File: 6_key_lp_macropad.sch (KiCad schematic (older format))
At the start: 9 parts, among them SW1 Rotary_Encoder_Switch, SW2 SW_Push, U1 ProMicro

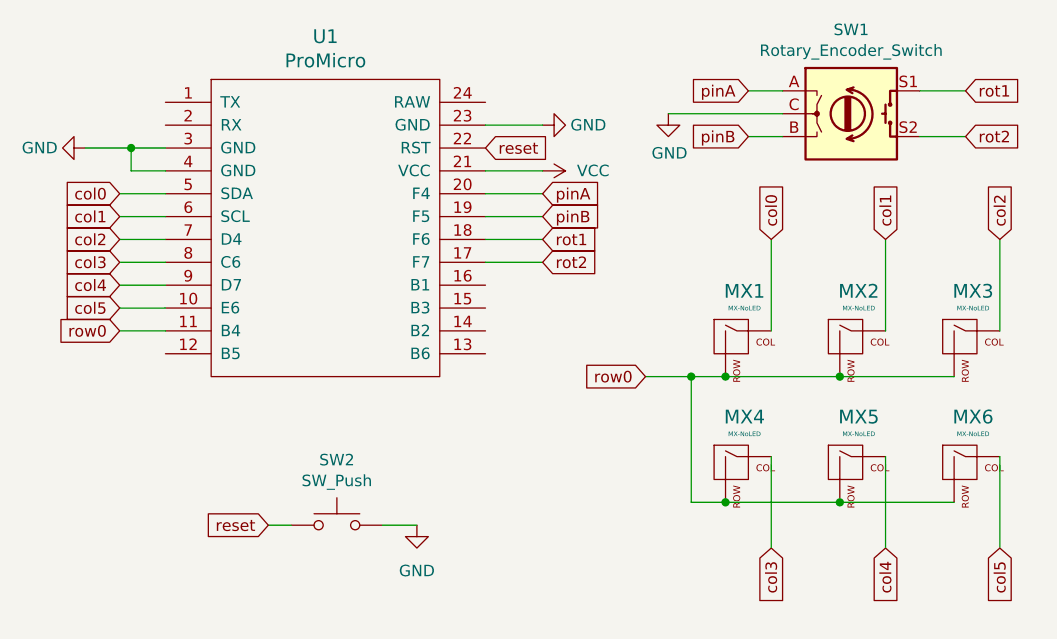
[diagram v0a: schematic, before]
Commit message: Made the first PCB version
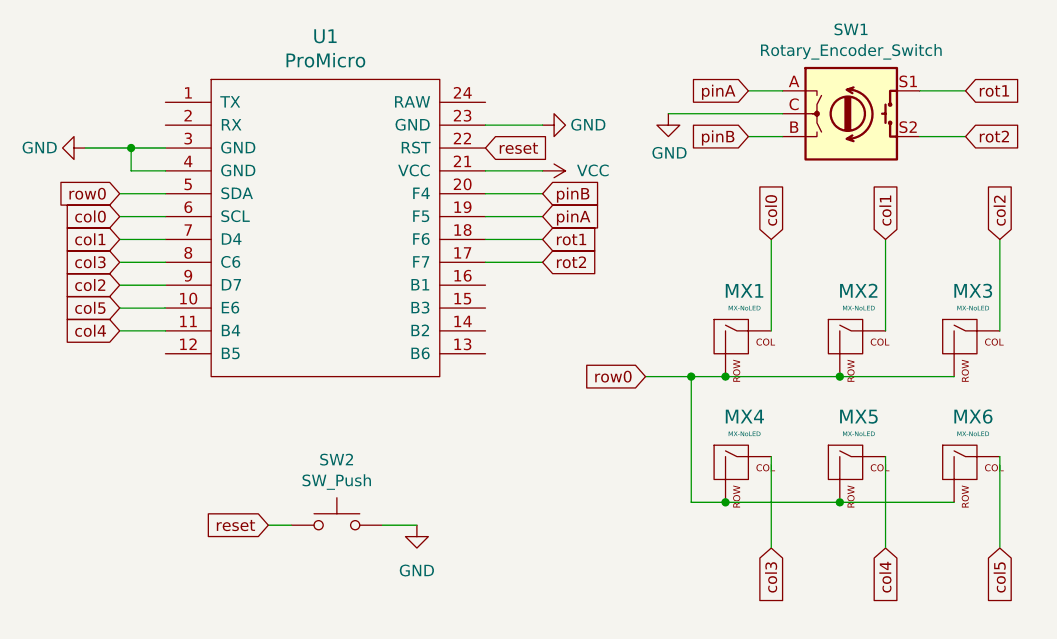
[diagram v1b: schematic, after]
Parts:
- U1: footprint promicro:ProMicro -> promicro:ProMicro-NoSilk
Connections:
- net col0: now also U1.6 (SCL); no longer U1.5 (SDA)
- net col1: now also U1.7 (D4); no longer U1.6 (SCL)
- net col2: now also U1.9 (D7); no longer U1.7 (D4)
- net col4: now also U1.11 (B4); no longer U1.9 (D7)
- net pinA: now also U1.19 (F5); no longer U1.20 (F4)
- net pinB: now also U1.20 (F4); no longer U1.19 (F5)
- net row0: now also U1.5 (SDA); no longer U1.11 (B4)
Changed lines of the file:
@@
 F 0 "U1" H 4900 4787 60  0000 C CNN
 F 1 "ProMicro" H 4900 4681 60  0000 C CNN
-F 2 "promicro:ProMicro" H 5000 2700 60  0001 C CNN
+F 2 "promicro:ProMicro-NoSilk" H 5000 2700 60  0001 C CNN
 F 3 "" H 5000 2700 60  0000 C CNN
 	1    4900 3750
@@
 Wire Wire Line
 	5600 3300 5850 3300
-Text GLabel 4000 3400 0    50   Input ~ 0
-col0
 Wire Wire Line
 	4200 3400 4000 3400
-Text GLabel 4000 3500 0    50   Input ~ 0
-col1
 Wire Wire Line
 	4200 3500 4000 3500
-Text GLabel 4000 3600 0    50   Input ~ 0
-col2
 Wire Wire Line
 	4200 3600 4000 3600
@@
 Text GLabel 5850 3600 2    50   Input ~ 0
 rot1
+Text GLabel 5850 3400 2    50   Input ~ 0
+pinB
 Text GLabel 5850 3500 2    50   Input ~ 0
-pinB
-Text GLabel 5850 3400 2    50   Input ~ 0
 pinA
-Text GLabel 4000 4000 0    50   Input ~ 0
-row0
 Wire Wire Line
 	5600 3400 5850 3400
@@
 Wire Wire Line
 	4650 4850 4750 4850
-Text GLabel 4000 3700 0    50   Input ~ 0
-col3
-Text GLabel 4000 3800 0    50   Input ~ 0
+Text GLabel 4000 4000 0    50   Input ~ 0
 col4
 Text GLabel 4000 3900 0    50   Input ~ 0
@@
 Wire Wire Line
 	6850 4950 6850 4550
+Text GLabel 4000 3400 0    50   Input ~ 0
+row0
+Text GLabel 4000 3700 0    50   Input ~ 0
+col3
+Text GLabel 4000 3800 0    50   Input ~ 0
+col2
+Text GLabel 4000 3600 0    50   Input ~ 0
+col1
+Text GLabel 4000 3500 0    50   Input ~ 0
+col0
 $EndSCHEMATC
